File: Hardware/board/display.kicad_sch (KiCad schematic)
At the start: 3 parts, among them U4 HC-FPC-0.5-40P-FH20, U5 PT4103B23F

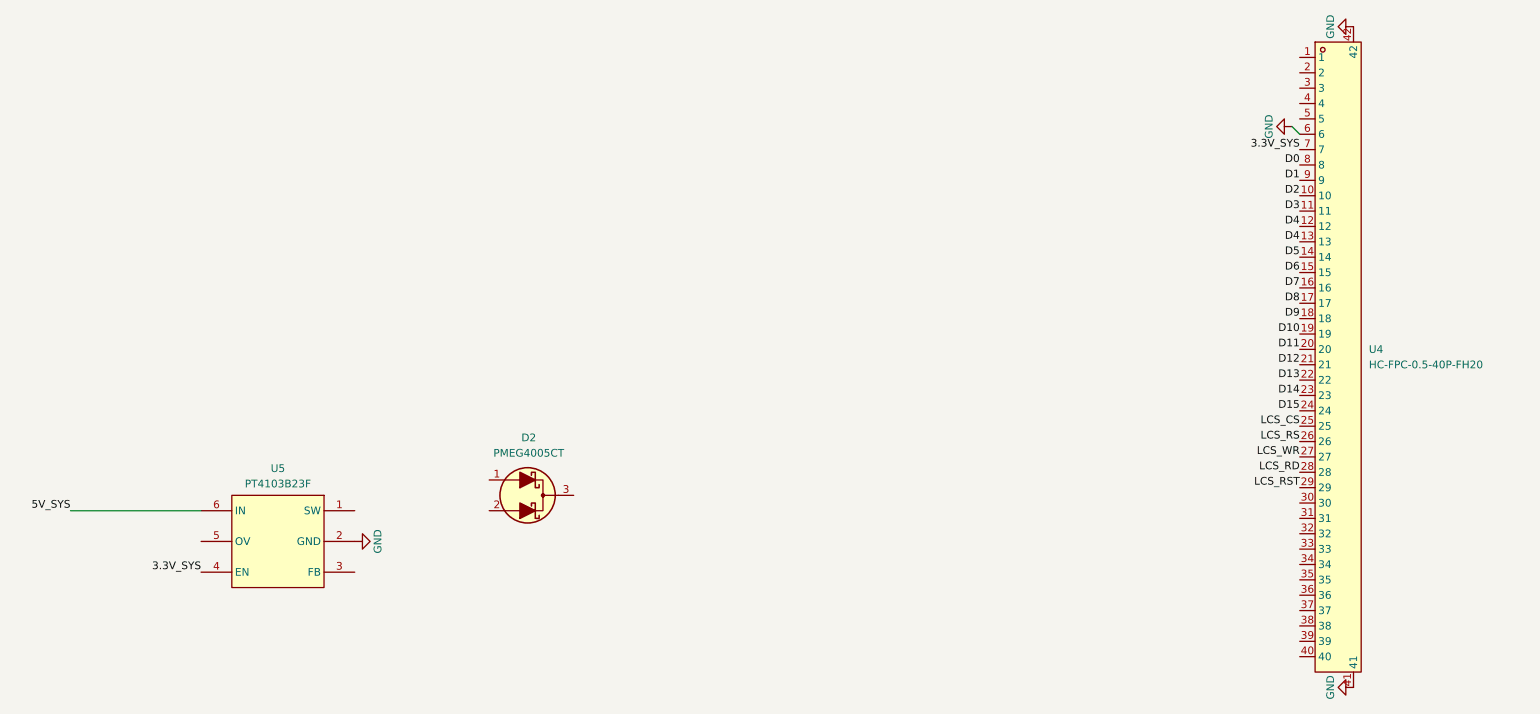
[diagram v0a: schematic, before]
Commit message: desigin designing
dsa
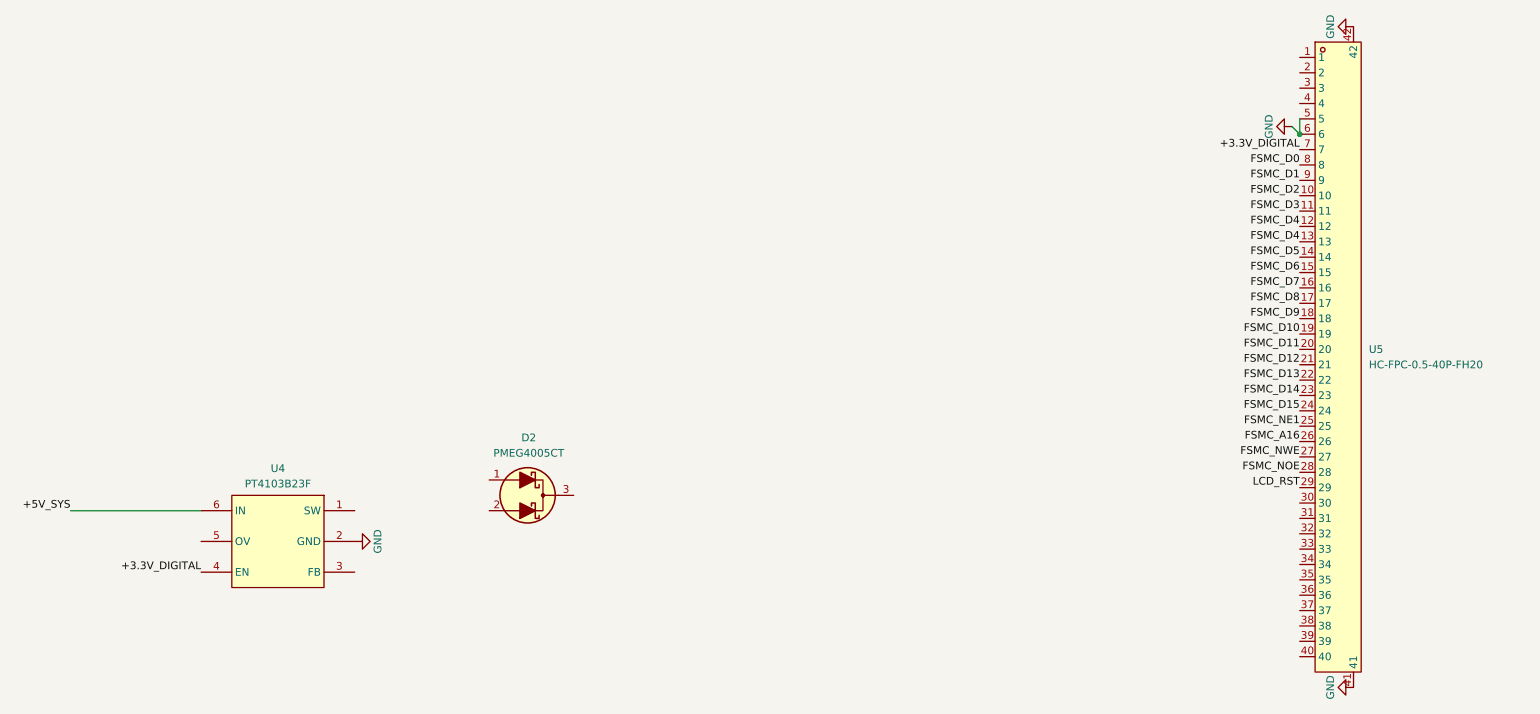
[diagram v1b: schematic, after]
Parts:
- renumbered U5 to U4, U4 to U5
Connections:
- net GND: now also U5.5
- net 3.3V_SYS renamed +3.3V_DIGITAL
- net 5V_SYS renamed +5V_SYS
- net D0 renamed FSMC_D0
- net D1 renamed FSMC_D1
- net D10 renamed FSMC_D10
- net D11 renamed FSMC_D11
- net D12 renamed FSMC_D12
- net D13 renamed FSMC_D13
- net D14 renamed FSMC_D14
- net D15 renamed FSMC_D15
- net D2 renamed FSMC_D2
- net D3 renamed FSMC_D3
- net D4 renamed FSMC_D4
- net D5 renamed FSMC_D5
- net D6 renamed FSMC_D6
- net D7 renamed FSMC_D7
- net D8 renamed FSMC_D8
- net D9 renamed FSMC_D9
- net LCS_CS renamed FSMC_NE1
- net LCS_RD renamed FSMC_NOE
- net LCS_RS renamed FSMC_A16
- net LCS_RST renamed LCD_RST
- net LCS_WR renamed FSMC_NWE
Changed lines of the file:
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@@
 	(generator_version "10.0")
 	(paper "A4")
+	(junction
+		(at 260.985 35.56)
+		(diameter 0)
+		(color 0 0 0 0)
+	)
 	(wire
 		(pts
@@
 		)
 	)
-	(label "D3"
+	(wire
+		(pts
+			(xy 260.985 33.02) (xy 260.985 35.56)
+		)
+		(stroke
+			(width 0)
+			(type default)
+		)
+	)
+	(label "FSMC_D3"
 		(at 260.985 48.26 180)
 		(effects
@@
 		)
 	)
-	(label "LCS_CS"
+	(label "FSMC_NE1"
 		(at 260.985 83.82 180)
 		(effects
@@
 		)
 	)
-	(label "3.3V_SYS"
+	(label "+3.3V_DIGITAL"
 		(at 260.985 38.1 180)
 		(effects
@@
 		)
 	)
-	(label "D1"
+	(label "FSMC_D1"
 		(at 260.985 43.18 180)
 		(effects
@@
 		)
 	)
-	(label "D13"
+	(label "FSMC_D13"
 		(at 260.985 76.2 180)
 		(effects
@@
 		)
 	)
-	(label "D14"
+	(label "FSMC_D14"
 		(at 260.985 78.74 180)
 		(effects
@@
 		)
 	)
-	(label "D10"
+	(label "FSMC_D10"
 		(at 260.985 68.58 180)
 		(effects
@@
 		)
 	)
-	(label "D12"
+	(label "FSMC_D12"
 		(at 260.985 73.66 180)
 		(effects
@@
 		)
 	)
-	(label "LCS_RS"
+	(label "FSMC_A16"
 		(at 260.985 86.36 180)
 		(effects
@@
 		)
 	)
-	(label "D11"
+	(label "FSMC_D11"
 		(at 260.985 71.12 180)
 		(effects
@@
 		)
 	)
-	(label "D5"
+	(label "FSMC_D5"
 		(at 260.985 55.88 180)
 		(effects
@@
 		)
 	)
-	(label "3.3V_SYS"
+	(label "+3.3V_DIGITAL"
 		(at 79.375 107.95 180)
 		(effects
@@
 		)
 	)
-	(label "D6"
+	(label "FSMC_D6"
 		(at 260.985 58.42 180)
 		(effects
@@
 		)
 	)
-	(label "D0"
+	(label "FSMC_D0"
 		(at 260.985 40.64 180)
 		(effects
@@
 		)
 	)
-	(label "LCS_RST"
+	(label "LCD_RST"
 		(at 260.985 93.98 180)
 		(effects
@@
 		)
 	)
-	(label "D9"
+	(label "FSMC_D9"
 		(at 260.985 66.04 180)
 		(effects
@@
 		)
 	)
-	(label "D15"
+	(label "FSMC_D15"
 		(at 260.985 81.28 180)
 		(effects
@@
 		)
 	)
-	(label "D2"
+	(label "FSMC_D2"
 		(at 260.985 45.72 180)
 		(effects
@@
 		)
 	)
-	(label "LCS_WR"
+	(label "FSMC_NWE"
 		(at 260.985 88.9 180)
 		(effects
@@
 		)
 	)
-	(label "5V_SYS"
+	(label "+5V_SYS"
 		(at 57.785 97.79 180)
 		(effects
@@
 		)
 	)
-	(label "D8"
+	(label "FSMC_D8"
 		(at 260.985 63.5 180)
 		(effects
@@
 		)
 	)
-	(label "D4"
+	(label "FSMC_D4"
 		(at 260.985 50.8 180)
 		(effects
@@
 		)
 	)
-	(label "D4"
+	(label "FSMC_D4"
 		(at 260.985 53.34 180)
 		(effects
@@
 		)
 	)
-	(label "LCS_RD"
+	(label "FSMC_NOE"
 		(at 260.985 91.44 180)
 		(effects
@@
 		)
 	)
-	(label "D7"
+	(label "FSMC_D7"
 		(at 260.985 60.96 180)
 		(effects
@@
 		(dnp no)
 		(fields_autoplaced yes)
-		(property "Reference" "#PWR020"
+		(property "Reference" "#PWR018"
 			(at 111.125 102.87 0)
 			(hide yes)
@@
 			(project "board"
 				(path "/a701f4fd-d5c8-4ab0-b464-3edf07ec58ed/a518d5fa-3e63-4101-a721-9b8ba5303779"
-					(reference "#PWR020")
+					(reference "#PWR018")
 					(unit 1)
 				)
@@
 		(in_pos_files yes)
 		(dnp no)
-		(property "Reference" "U5"
+		(property "Reference" "U4"
 			(at 92.075 90.805 0)
 			(show_name no)
@@
 			(project "board"
 				(path "/a701f4fd-d5c8-4ab0-b464-3edf07ec58ed/a518d5fa-3e63-4101-a721-9b8ba5303779"
-					(reference "U5")
+					(reference "U4")
 					(unit 1)
 				)
@@
 		(dnp no)
 		(fields_autoplaced yes)
-		(property "Reference" "U4"
+		(property "Reference" "U5"
 			(at 272.415 71.1199 0)
 			(show_name no)
@@
 			(project "board"
 				(path "/a701f4fd-d5c8-4ab0-b464-3edf07ec58ed/a518d5fa-3e63-4101-a721-9b8ba5303779"
-					(reference "U4")
+					(reference "U5")
 					(unit 1)
 				)
@@
 		(dnp no)
 		(fields_autoplaced yes)
-		(property "Reference" "#PWR018"
+		(property "Reference" "#PWR020"
 			(at 263.525 17.78 0)
 			(hide yes)
@@
 			(project "board"
 				(path "/a701f4fd-d5c8-4ab0-b464-3edf07ec58ed/a518d5fa-3e63-4101-a721-9b8ba5303779"
-					(reference "#PWR018")
+					(reference "#PWR020")
 					(unit 1)
 				)
@@
 		(dnp no)
 		(fields_autoplaced yes)
-		(property "Reference" "#PWR017"
+		(property "Reference" "#PWR021"
 			(at 263.525 127 0)
 			(hide yes)
@@
 			(project "board"
 				(path "/a701f4fd-d5c8-4ab0-b464-3edf07ec58ed/a518d5fa-3e63-4101-a721-9b8ba5303779"
-					(reference "#PWR017")
+					(reference "#PWR021")
 					(unit 1)
 				)

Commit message: sdadsa
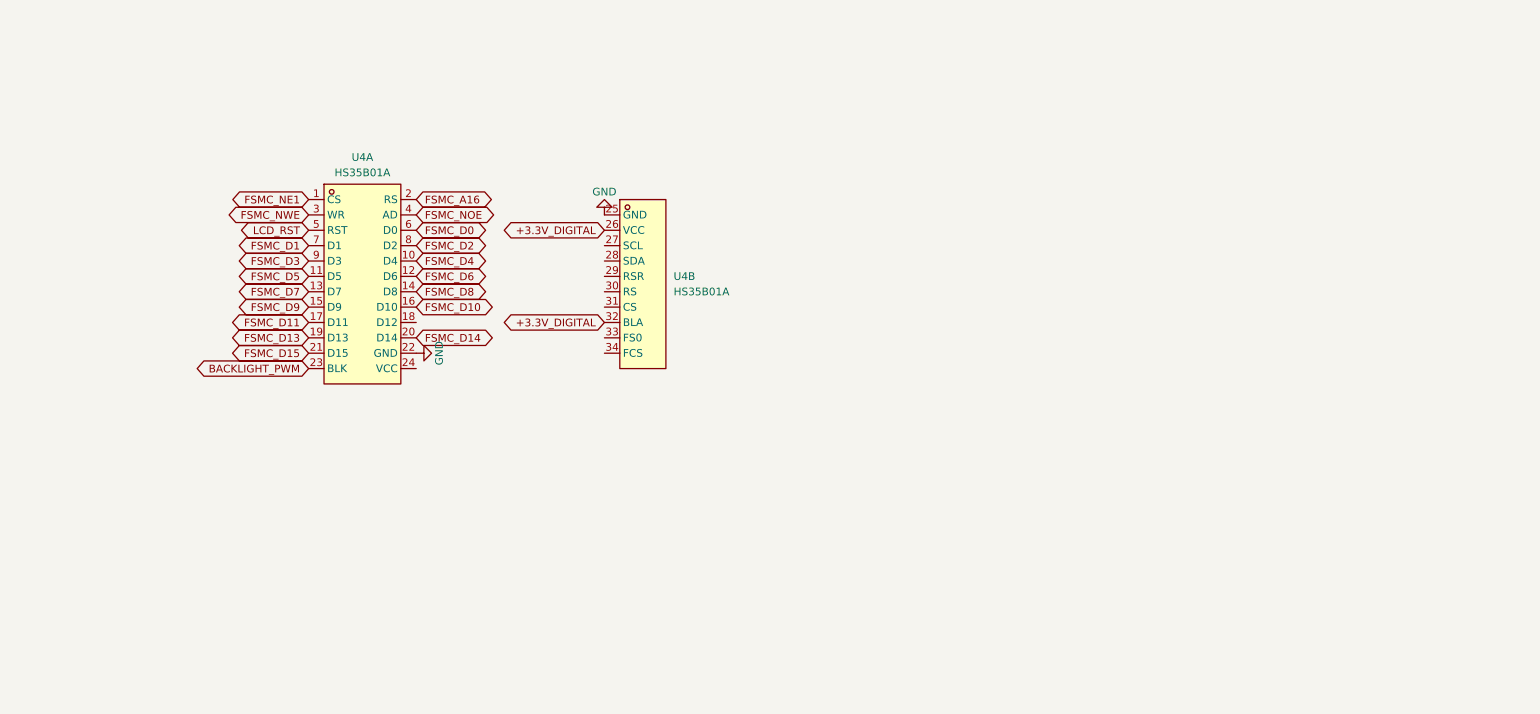
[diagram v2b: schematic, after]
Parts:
- removed D2: PMEG4005CT, PCM_Package_TO_SOT_SMD_AKL:SOT-23, symbol PCM_Diode_Schottky_AKL:PMEG4005CT
- removed U4: PT4103B23F, easyeda_imports:SOT-23-6_L2.9-W1.6-P0.95-LS2.8-BR, symbol easyeda_imports:PT4103B23F
- removed U5: HC-FPC-0.5-40P-FH20, easyeda_imports:FPC-SMD_40P-P0.50_HC-FPC-0.5-40P-FH20, symbol easyeda_imports:HC-FPC-0.5-40P-FH20
- added U4: HS35B01A, easyeda_imports:LCD-TH_L96.5-W57.3_HS35B01A, symbol easyeda_imports:HS35B01A
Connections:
- net +3.3V_DIGITAL: now also U4.26 (VCC), U4.32 (BLA)
- net FSMC_A16: now also U4.2 (RS)
- net FSMC_D0: now also U4.6 (D0)
- net FSMC_D1: now also U4.7 (D1)
- net FSMC_D10: now also U4.16 (D10)
- net FSMC_D11: now also U4.17 (D11)
- net FSMC_D13: now also U4.19 (D13)
- net FSMC_D14: now also U4.20 (D14)
- net FSMC_D15: now also U4.21 (D15)
- net FSMC_D2: now also U4.8 (D2)
- net FSMC_D3: now also U4.9 (D3)
- net FSMC_D4: now also U4.10 (D4)
- net FSMC_D5: now also U4.11 (D5)
- net FSMC_D6: now also U4.12 (D6)
- net FSMC_D7: now also U4.13 (D7)
- net FSMC_D8: now also U4.14 (D8)
- net FSMC_D9: now also U4.15 (D9)
- net FSMC_NE1: now also U4.1 (CS)
- net FSMC_NOE: now also U4.4 (AD)
- net FSMC_NWE: now also U4.3 (WR)
- net GND: now also U4.22 (GND), U4.25 (GND)
- net LCD_RST: now also U4.5 (RST)
- new net BACKLIGHT_PWM: U4.23 (BLK)
